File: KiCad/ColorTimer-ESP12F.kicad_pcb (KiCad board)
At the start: 2 copper layers, 72 x 47 mm, 40 parts, among them J1 SW_CON, J2 USB_B_Micro, J3 COLOER_LED, J4 AkitsukiCON, J5 GPIO_CON, J6 POWER_CON, Q1 2N7000, Q2 2N7000, SW1 RESET, SW2 Trigger SW, SW3 FLASH, SW4 SW_SPDT, U1 ESP-12F, U2 CH340K, U3 BA033CC0T_TO220

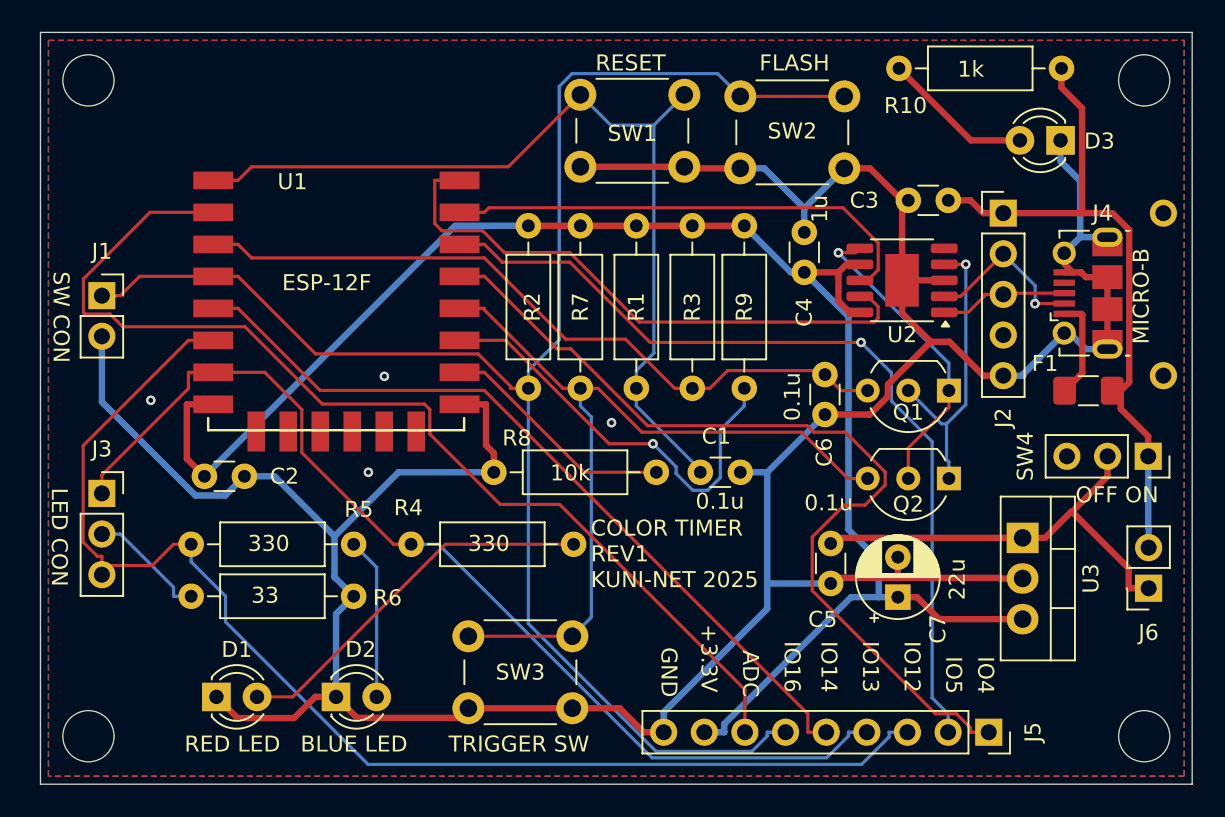
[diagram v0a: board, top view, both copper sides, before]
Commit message: 表面実装部品版 作成開始
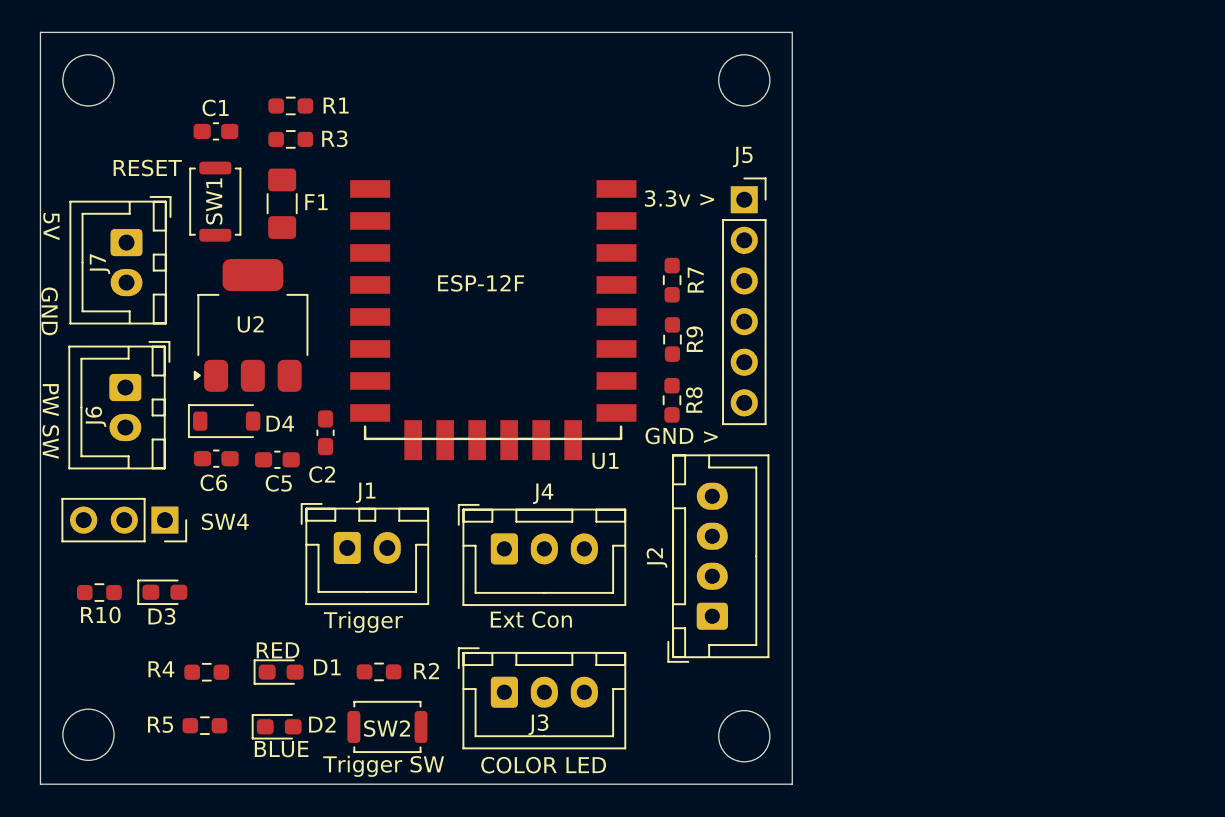
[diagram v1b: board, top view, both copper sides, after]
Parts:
- removed C3: 10u, Capacitor_THT:C_Disc_D3.0mm_W1.6mm_P2.50mm
- removed C4: 1u, Capacitor_THT:C_Disc_D3.0mm_W1.6mm_P2.50mm
- removed C7: 22u, Capacitor_THT:CP_Radial_D5.0mm_P2.50mm
- removed Q1, Q2: 2N7000, Package_TO_SOT_THT:TO-92_Inline_Wide
- removed R6: 33, Resistor_THT:R_Axial_DIN0207_L6.3mm_D2.5mm_P10.16mm_Horizontal
- removed SW3: FLASH, Button_Switch_THT:SW_PUSH_6mm_H8mm
- removed U3: BA033CC0T_TO220, Package_TO_SOT_THT:TO-220-3_Vertical
- added D4: D_Schottky, Diode_SMD:D_SOD-123, F.Cu at (106.6, 64.3)
- added J7: POWER_CON, Connector_JST:JST_XH_B2B-XH-A_1x02_P2.50mm_Vertical, F.Cu at (100.4, 53.1)
- C1, C2: footprint Capacitor_THT:C_Disc_D3.0mm_W1.6mm_P2.50mm -> Capacitor_SMD:C_0603_1608Metric_Pad1.08x0.95mm_HandSolder
- C5, C6: value 0.1u -> 22u; footprint Capacitor_THT:C_Disc_D3.0mm_W1.6mm_P2.50mm -> Capacitor_SMD:C_0603_1608Metric_Pad1.08x0.95mm_HandSolder
- D1, D2, D3: footprint LED_THT:LED_D3.0mm -> LED_SMD:LED_0603_1608Metric_Pad1.05x0.95mm_HandSolder
- J1: footprint Connector_PinSocket_2.54mm:PinSocket_1x02_P2.54mm_Vertical -> Connector_JST:JST_XH_B2B-XH-A_1x02_P2.50mm_Vertical
- J2: value USB_B_Micro -> OLED; footprint Connector_USB:USB_Micro-B_Molex-105017-0001 -> Connector_JST:JST_XH_B4B-XH-A_1x04_P2.50mm_Vertical
- J3: footprint Connector_PinSocket_2.54mm:PinSocket_1x03_P2.54mm_Vertical -> Connector_JST:JST_XH_B3B-XH-A_1x03_P2.50mm_Vertical
- J4: value AkitsukiCON -> Ext_Con; footprint AE:AE-USB-MICRO-B-D -> Connector_JST:JST_XH_B3B-XH-A_1x03_P2.50mm_Vertical
- J5: value GPIO_CON -> Downloader_CON; footprint Connector_PinSocket_2.54mm:PinSocket_1x09_P2.54mm_Vertical -> Connector_PinSocket_2.54mm:PinSocket_1x06_P2.54mm_Vertical
- J6: value POWER_CON -> POWER_SW_CON; footprint Connector_PinSocket_2.54mm:PinSocket_1x02_P2.54mm_Vertical -> Connector_JST:JST_XH_B2B-XH-A_1x02_P2.50mm_Vertical
- R1, R10, R2, R3, R7, R8, R9: footprint Resistor_THT:R_Axial_DIN0207_L6.3mm_D2.5mm_P10.16mm_Horizontal -> Resistor_SMD:R_0603_1608Metric_Pad0.98x0.95mm_HandSolder
- R4, R5: value 330 -> 1k; footprint Resistor_THT:R_Axial_DIN0207_L6.3mm_D2.5mm_P10.16mm_Horizontal -> Resistor_SMD:R_0603_1608Metric_Pad0.98x0.95mm_HandSolder
- SW1, SW2: footprint Button_Switch_THT:SW_PUSH_6mm_H8mm -> Button_Switch_SMD:SW_Push_SPST_NO_Alps_SKRK
- U2: value CH340K -> AMS1117-3.3; footprint Package_SO:SSOP-10-1EP_3.9x4.9mm_P1mm_EP2.1x3.3mm -> Package_TO_SOT_SMD:SOT-223-3_TabPin2
- moved H3 77.7 mm to (98.0, 83.9)
- moved J6 65.2 mm to (100.3, 62.2), turned to -90 degrees
- moved D3 62.7 mm to (102.8, 75.0), turned to 0 degrees
- moved SW4 61.6 mm to (102.8, 70.5)
- moved R10 59.8 mm to (98.7, 75.0)
- moved H2 58.0 mm to (139.0, 43.0)
- moved F1 51.7 mm to (110.1, 50.7), turned to -90 degrees
- moved SW2 45.1 mm to (116.7, 83.4), turned to 0 degrees
- moved U2 40.7 mm to (108.3, 58.3), turned to 90 degrees
- moved J4 39.9 mm to (124.0, 72.3)
- moved C6 38.4 mm to (106.0, 66.6), turned to 0 degrees
- moved C1 37.0 mm to (106.0, 46.2)
- moved J5 36.6 mm to (139.0, 50.5), turned to 0 degrees
- moved C5 35.0 mm to (109.8, 66.7), turned to 180 degrees
- moved J2 31.0 mm to (137.0, 76.5)
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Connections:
- C6 pad 1: EN -> +3.3V
- F1 pad 1: Net-(J2-VBUS) -> Net-(J7-Pin_1)
- J1 pad 1: /GPIO16 -> Net-(J1-Pin_1)
- J2 pad 1: Net-(J2-VBUS) -> /GPIO4
- J2 pad 2: Net-(J2-D-) -> /GPIO5
- J2 pad 3: Net-(J2-D+) -> +3.3V
- J2 pad 4: unconnected-(J2-ID-Pad4) -> GND
- J3 pad 1: /GPIO13 -> Net-(J3-Pin_1)
- J3 pad 2: Net-(J3-Pin_2) -> GND
- J3 pad 3: /GPIO12 -> Net-(J3-Pin_3)
- J4 pad 1: VCC -> /GPIO14
- J4 pad 2: Net-(J2-D-) -> /ADC
- J4 pad 3: Net-(J2-D+) -> GND
- J5 pad 1: /GPIO4 -> +3.3V
- J5 pad 2: /GPIO5 -> TxD
- J5 pad 3: /GPIO12 -> RxD
- J5 pad 4: /GPIO13 -> EN
- J5 pad 5: /GPIO14 -> GPIO0
- J5 pad 6: /GPIO16 -> GND
- R10 pad 2: VCC -> +5V
- R2 pad 2: /GPIO16 -> Net-(J1-Pin_1)
- R4 pad 2: /GPIO13 -> Net-(J3-Pin_1)
- R5 pad 2: /GPIO12 -> Net-(J3-Pin_3)
- SW2 pad 2: /GPIO16 -> Net-(J1-Pin_1)
- U1 pad 4: /GPIO16 -> Net-(J1-Pin_1)
- U1 pad 6: /GPIO12 -> Net-(J3-Pin_3)
- U1 pad 7: /GPIO13 -> Net-(J3-Pin_1)
- U2 pad 1: Net-(J2-D+) -> GND
- U2 pad 2: Net-(J2-D-) -> Net-(D4-A)
- U2 pad 3: GND -> +5V
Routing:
- net GND: track 205.0 -> 0.00 mm, vias 4 -> 0
- net +3.3V: track 106.1 -> 0.00 mm
- net /GPIO16: track 103.3 -> 0.00 mm
- net /GPIO12: track 79.5 -> 0.00 mm
- net /ADC: track 67.3 -> 0.00 mm
- net /GPIO13: track 64.6 -> 0.00 mm
- net /GPIO4: track 57.3 -> 0.00 mm
- net Net-(U1-REST): track 56.4 -> 0.00 mm
- net /GPIO5: track 55.0 -> 0.00 mm, vias 1 -> 0
- net GPIO0: track 53.5 -> 0.00 mm
- net /GPIO14: track 49.3 -> 0.00 mm
- net EN: track 44.9 -> 0.00 mm
- net VCC: track 43.0 -> 0.00 mm
- net TxD: track 36.0 -> 0.00 mm
- net RxD: track 31.0 -> 0.00 mm
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- removed copper zone on B.Cu, net GND
- removed copper zone on F.Cu, net GND
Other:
- board size 72 x 47 mm -> 47 x 47 mm
- board text added: "+3.3v"
- board text added: "3.3v >"
- board text added: "5V"
- board text added: "BLUE"
- board text added: "COLOR LED"
- board text added: "EN"
- board text added: "Ext Con"
- board text added: "GND >"
- board text added: "GPIO0"
- board text added: "PW SW"
- board text added: "RED"
- board text added: "RxD->TxD"
- board text added: "Trigger"
- board text added: "Trigger SW"
- board text added: "TxD->RxD"
- board text removed: "+3.3V"
- board text removed: "0.1u"
- board text removed: "10k"
- board text removed: "1k"
- board text removed: "1u"
- board text removed: "22u"
- board text removed: "33"
- board text removed: "330"
- board text removed: "ADC"
- board text removed: "BLUE LED"
- board text removed: "COLOR TIMER REV1 KUNI-NET 2025"
- board text removed: "FLASH"
- board text removed: "IO12"
- board text removed: "IO13"
- board text removed: "IO14"
- board text removed: "IO16"
- board text removed: "IO4"
- board text removed: "IO5"
- board text removed: "LED CON"
- board text removed: "MICRO-B"
- board text removed: "OFF ON"
- board text removed: "RED LED"
- board text removed: "SW CON"
- board text removed: "TRIGGER SW"
